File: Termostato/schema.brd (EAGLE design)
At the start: 108.9 x 87.6 mm, 11 parts, among them K1 RELAY-SPDT-JZC-11F

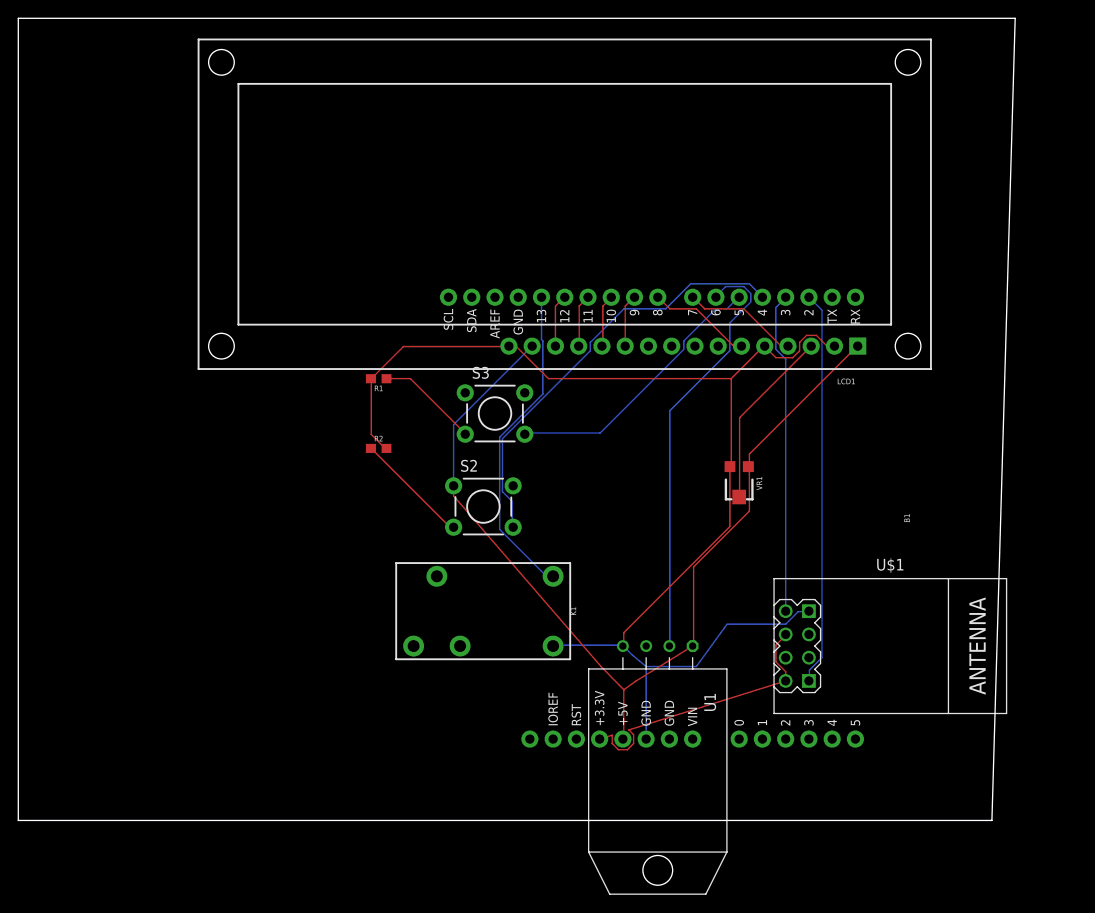
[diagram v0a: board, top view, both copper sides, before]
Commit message: Updated board design
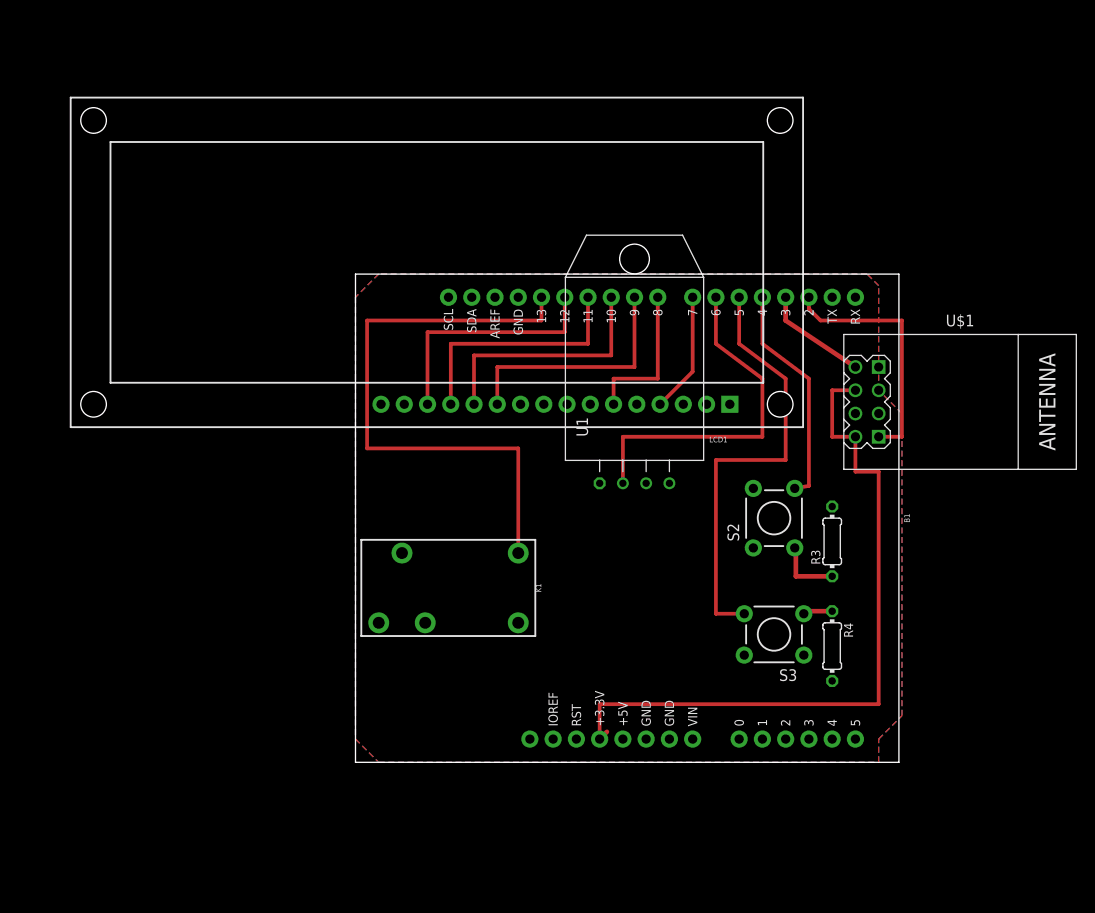
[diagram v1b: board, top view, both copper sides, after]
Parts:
- removed R1, R2: 220, SparkFun-Resistors:0603
- removed VR1: 10k, SparkFun-Resistors:TRIMPOT-SMD-TC33X
- added R3, R4: 220, resistor:0204/7
- moved S3 38.9 mm to (82.5, 14.0), turned to 180 degrees
- moved S2 31.8 mm to (82.5, 26.7), turned to 90 degrees
- moved U$1 27.7 mm to (102.9, 39.4)
- moved U1 18.0 mm to (67.3, 30.5), turned to 0 degrees
- moved LCD1 15.3 mm to (45.7, 54.6)
- moved K1 4.58 mm to (45.7, 19.1)
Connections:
- removed net N$1: LCD1.3, VR1.2
- net GND: now also R3.2, R4.2; no longer R1.2, R2.2, VR1.3
- net N$2: now also R3.1; no longer R2.1
- net N$4: now also R4.1; no longer R1.1
- net VCC: no longer VR1.1
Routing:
- net GND: track 139.9 -> 0.00 mm
- net VCC: track 102.7 -> 0.00 mm
- net 3.3V: track 30.9 -> 77.3 mm
- net D13: track 35.4 -> 63.5 mm
- net TX: track 35.2 -> 11.7 mm
- net D4: track 46.7 -> 24.8 mm
- net D11: track 5.75 -> 26.7 mm
- net D10: track 5.76 -> 26.7 mm
- net D9: track 5.78 -> 26.7 mm
- net D12: track 5.78 -> 26.7 mm
- net N$1: track 19.7 -> 0.00 mm
- net D5: track 30.2 -> 47.8 mm
- net RX: track 43.1 -> 27.2 mm
- net N$3: track 46.8 -> 38.1 mm
- net N$4: track 11.1 -> 3.32 mm
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- added copper zone on layer 16, net GND
- added copper zone on layer 1, net VCC
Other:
- board size 108.9 x 87.6 mm -> 59.4 x 53.3 mm
